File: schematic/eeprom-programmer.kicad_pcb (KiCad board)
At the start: 2 copper layers, 8 parts, among them IC1 AT28C64B-15PU, U1 74HC595, U2 74HC595

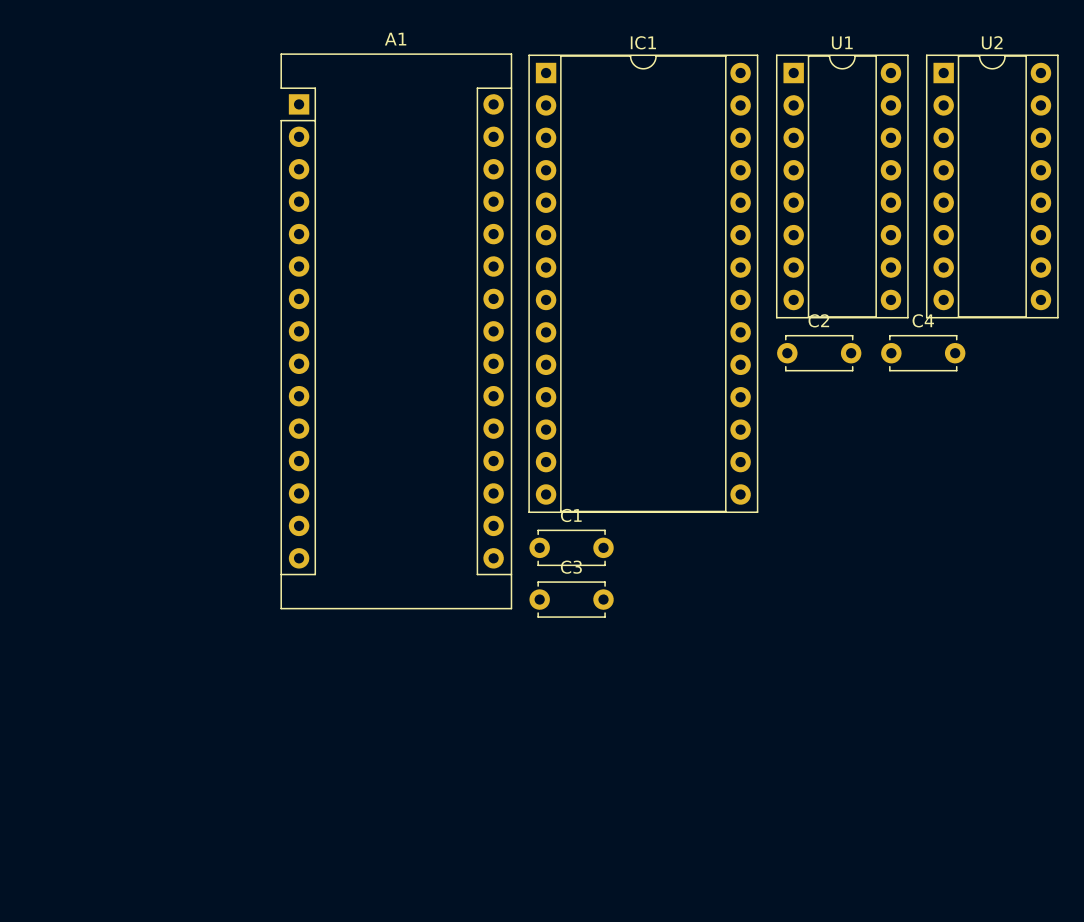
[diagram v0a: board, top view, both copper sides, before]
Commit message: Rearrange parts
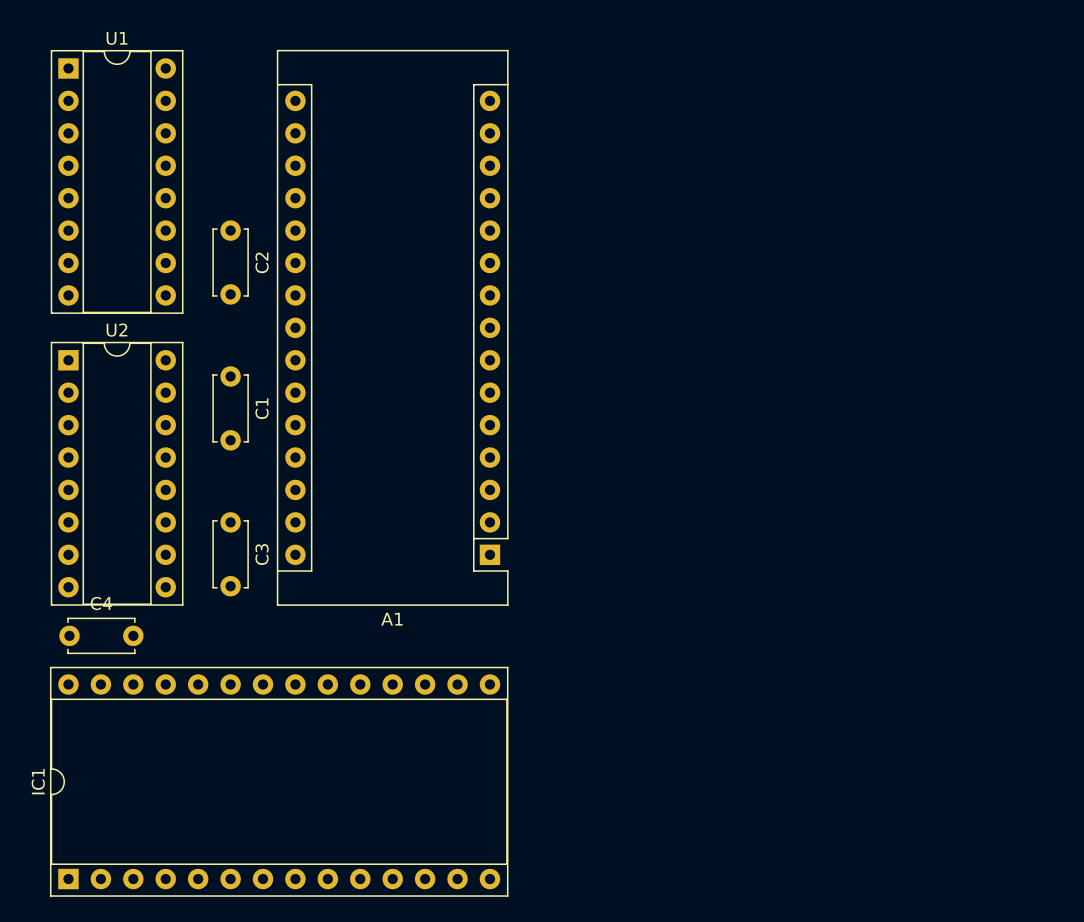
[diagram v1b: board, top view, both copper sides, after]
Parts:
- moved IC1 73.4 mm to (95.2, 133.3), turned to 90 degrees
- moved U2 72.2 mm to (95.2, 92.7)
- moved C4 68.1 mm to (95.3, 114.3)
- moved U1 56.8 mm to (95.2, 69.8)
- moved C2 44.7 mm to (108.0, 82.5), turned to 270 degrees
- moved A1 38.3 mm to (128.3, 108.0), turned to 180 degrees
- moved C1 27.7 mm to (108.0, 94.0), turned to 270 degrees
- moved C3 25.0 mm to (108.0, 105.4), turned to 270 degrees
